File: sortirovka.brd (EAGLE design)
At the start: 86.8 x 85.8 mm, 72 parts, among them IC1 DS1307Z, IC3 LM1117IMPX-3.3, U1 MAX3485CSA, X1 PI3-CON, X10 MKDSN1,5/3-5,08, X3 MKDSN1,5/4-5,08, X4 MKDSN1,5/2-5,08, X5 22-23-2021, X6 22-23-2051, X7 22-23-2041, X8 22-23-2051, X9 MKDSN1,5/7-5,08

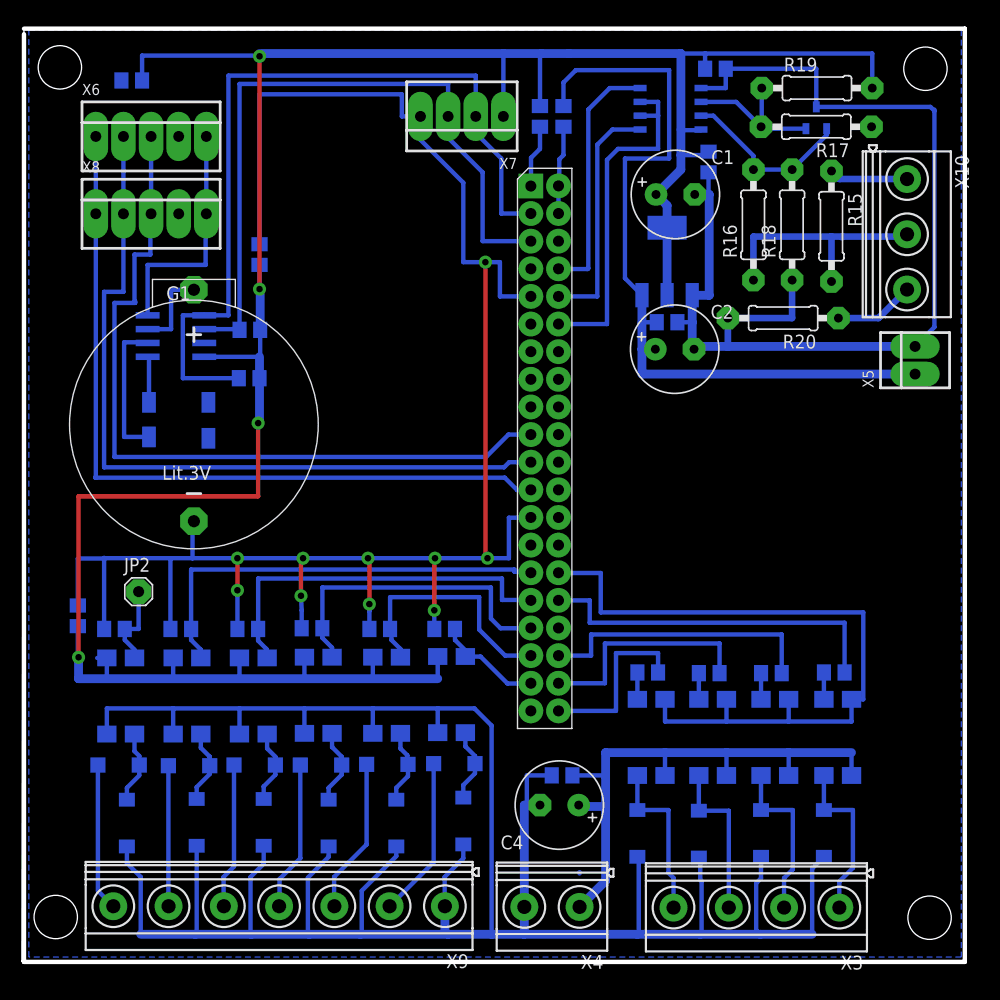
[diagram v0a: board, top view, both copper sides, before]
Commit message: rev 1.1 to produce
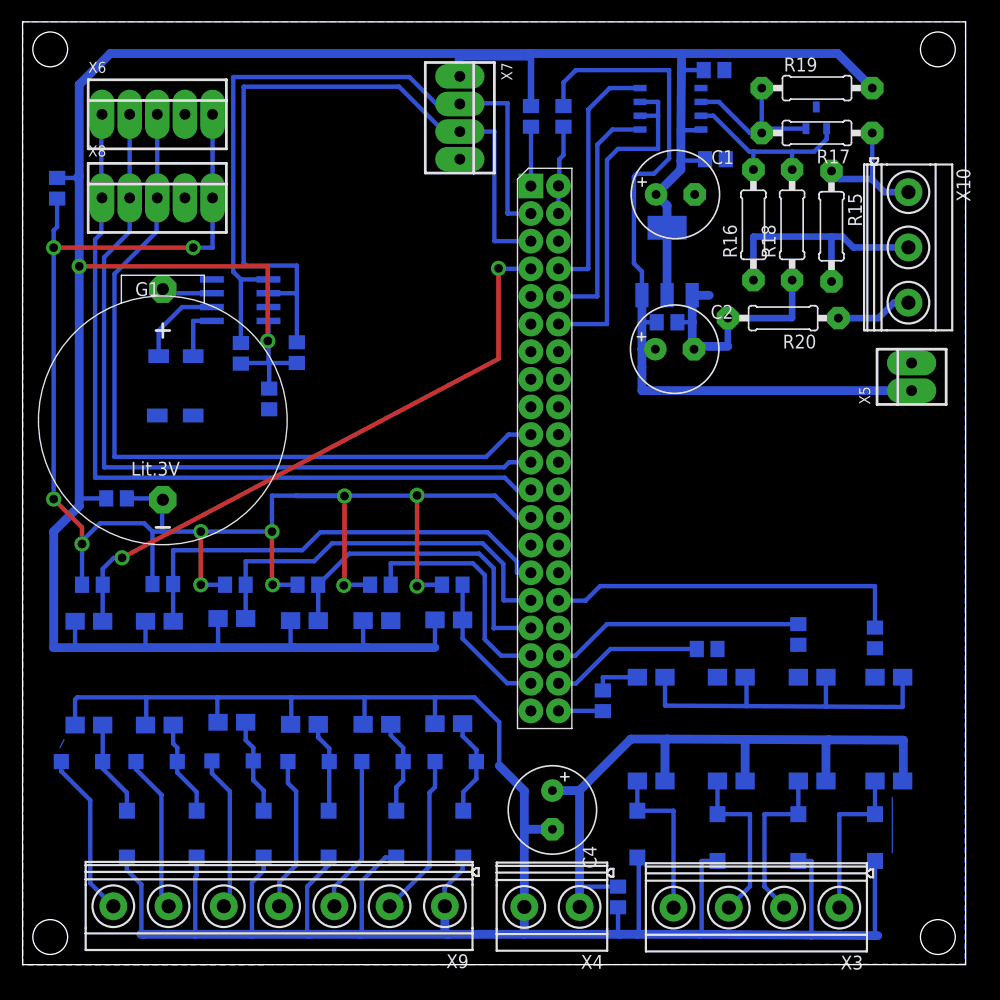
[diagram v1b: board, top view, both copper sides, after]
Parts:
- removed JP2: (no value), pinhead:1X01
- OC1, OC10, OC2, OC3, OC4, OC5, OC6, OC7, OC8, OC9: device MyLib:SMD4 -> MyLib:SFH6106
- R16, R17: value 47 -> 15
- R18, R19: value 560 -> 1k5
- R20: value 560 -> 10
- moved C5 13.3 mm to (20.1, 47.2), turned to 270 degrees
- moved C6 12.3 mm to (52.2, 1.46), turned to 270 degrees
- moved C8 12.0 mm to (0.64, 66.6), turned to 270 degrees
- moved C9 11.4 mm to (6.10, 38.1), turned to 180 degrees
- moved IC1 6.77 mm to (17.5, 56.3)
- moved R4 4.91 mm to (75.8, 25.3), turned to 90 degrees
- moved R1 4.88 mm to (50.8, 19.5), turned to 270 degrees
- moved R10 4.80 mm to (22.7, 51.5), turned to 270 degrees
- moved OC10 4.76 mm to (77.1, 16.9)
- moved D4 4.71 mm to (75.8, 6.92)
- moved R5 4.54 mm to (3.87, 30.2)
- moved R6 4.45 mm to (10.4, 30.2)
- moved R3 4.33 mm to (68.8, 25.6), turned to 90 degrees
- moved R8 4.22 mm to (17.0, 30.2)
- moved R13 4.12 mm to (37.0, 30.2)
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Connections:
- net N$43: no longer JP2.1
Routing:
- net GND: track 365.9 -> 217.7 mm, vias 10 -> 12
- net N$43: track 7.73 -> 57.5 mm, vias 0 -> 2
- net +3V3: track 243.3 -> 262.8 mm, vias 4 -> 2
- net N$6: track 16.2 -> 4.10 mm
- net +24V: track 52.0 -> 64.0 mm
- net N$27: track 76.3 -> 65.8 mm
- net N$7: track 21.2 -> 14.1 mm
- net GND1: track 232.6 -> 225.8 mm
- net N$44: track 0.00 -> 5.08 mm
- net N$25: track 13.2 -> 8.14 mm
- net N$46: track 7.25 -> 12.2 mm
- net N$26: track 65.2 -> 69.0 mm
- net N$34: track 10.0 -> 12.9 mm
- net N$8: track 26.0 -> 23.3 mm
- net N$20: track 7.87 -> 5.21 mm
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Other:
- board size 86.8 x 85.8 mm -> 86.7 x 86.7 mm
